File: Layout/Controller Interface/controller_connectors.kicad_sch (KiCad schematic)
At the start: 16 parts, among them J2 Controller 2, J3 Controller 3, J4 Controller 4, J7 Controller 1

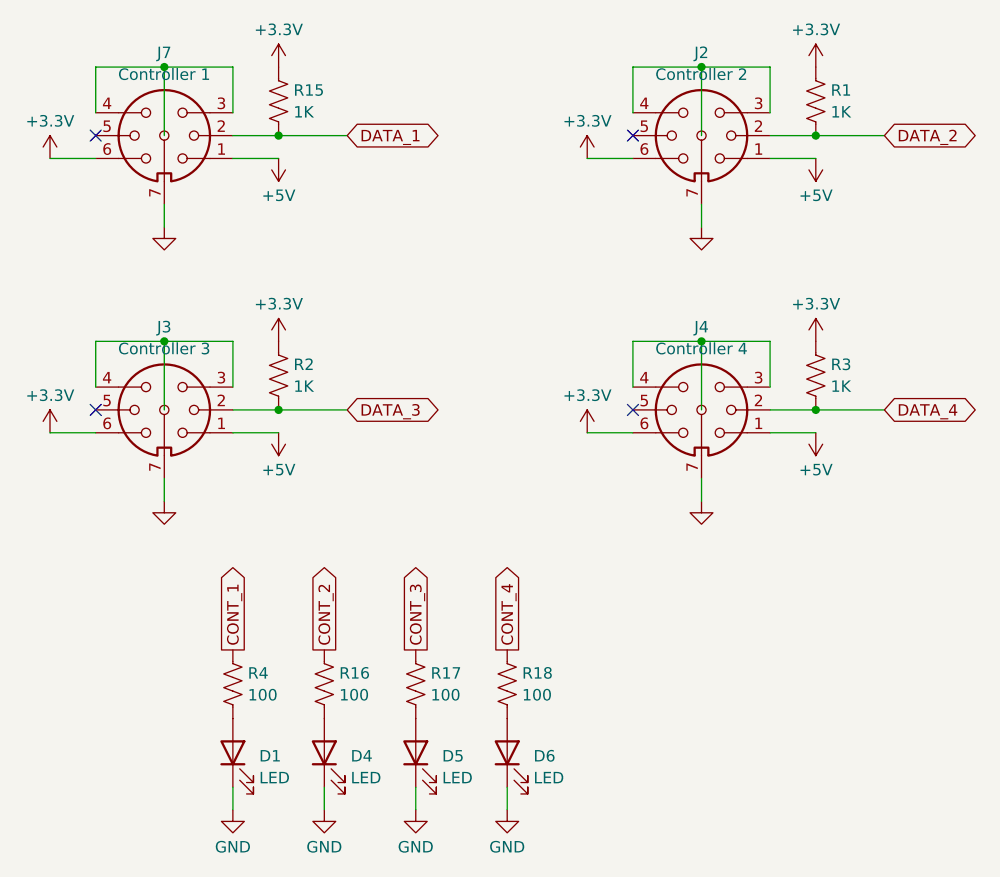
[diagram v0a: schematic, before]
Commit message: Completed schematic and layout
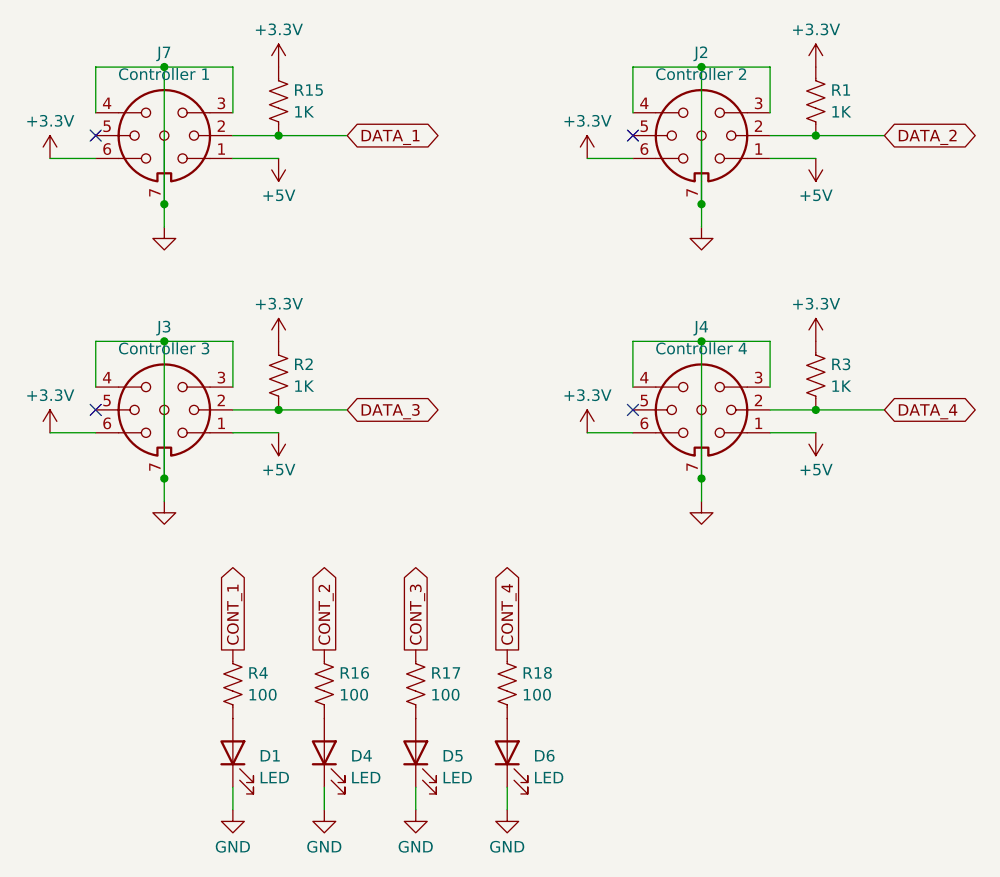
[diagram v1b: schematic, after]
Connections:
- net GND: now also J2.3, J2.4, J3.3, J3.4, J4.3, J4.4, J7.3, J7.4
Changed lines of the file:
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@@
 (kicad_sch (version 20230121) (generator eeschema)
   (paper "A4")
+  (junction (at 110.49 82.55) (diameter 0) (color 0 0 0 0)
+  )
+  (junction (at 170.18 82.55) (diameter 0) (color 0 0 0 0)
+  )
   (junction (at 123.19 105.41) (diameter 0) (color 0 0 0 0)
   )
-  (junction (at 170.18 97.79) (diameter 0) (color 0 0 0 0)
+  (junction (at 110.49 113.03) (diameter 0) (color 0 0 0 0)
   )
   (junction (at 110.49 97.79) (diameter 0) (color 0 0 0 0)
+  )
+  (junction (at 170.18 97.79) (diameter 0) (color 0 0 0 0)
   )
   (junction (at 110.49 67.31) (diameter 0) (color 0 0 0 0)
@@
   )
   (junction (at 170.18 67.31) (diameter 0) (color 0 0 0 0)
+  )
+  (junction (at 170.18 113.03) (diameter 0) (color 0 0 0 0)
   )
   (no_connect (at 102.87 105.41))
@@
     (stroke (width 0) (type default))
   )
-  (wire (pts (xy 110.49 67.31) (xy 118.11 67.31))
+  (wire (pts (xy 102.87 67.31) (xy 110.49 67.31))
     (stroke (width 0) (type default))
   )
@@
     (stroke (width 0) (type default))
   )
-  (wire (pts (xy 170.18 97.79) (xy 170.18 105.41))
-    (stroke (width 0) (type default))
-  )
   (wire (pts (xy 177.8 105.41) (xy 182.88 105.41))
     (stroke (width 0) (type default))
@@
     (stroke (width 0) (type default))
   )
-  (wire (pts (xy 110.49 97.79) (xy 118.11 97.79))
-    (stroke (width 0) (type default))
-  )
-  (wire (pts (xy 102.87 67.31) (xy 110.49 67.31))
+  (wire (pts (xy 102.87 97.79) (xy 110.49 97.79))
     (stroke (width 0) (type default))
   )
@@
     (stroke (width 0) (type default))
   )
-  (wire (pts (xy 110.49 67.31) (xy 110.49 74.93))
+  (wire (pts (xy 110.49 113.03) (xy 110.49 115.57))
+    (stroke (width 0) (type default))
+  )
+  (wire (pts (xy 110.49 67.31) (xy 118.11 67.31))
     (stroke (width 0) (type default))
   )
   (wire (pts (xy 118.11 147.32) (xy 118.11 149.86))
+    (stroke (width 0) (type default))
+  )
+  (wire (pts (xy 110.49 67.31) (xy 110.49 82.55))
     (stroke (width 0) (type default))
   )
@@
   )
   (wire (pts (xy 182.88 105.41) (xy 190.5 105.41))
-    (stroke (width 0) (type default))
-  )
-  (wire (pts (xy 170.18 67.31) (xy 170.18 74.93))
-    (stroke (width 0) (type default))
-  )
-  (wire (pts (xy 110.49 113.03) (xy 110.49 115.57))
     (stroke (width 0) (type default))
   )
@@
     (stroke (width 0) (type default))
   )
-  (wire (pts (xy 110.49 97.79) (xy 110.49 105.41))
-    (stroke (width 0) (type default))
-  )
   (wire (pts (xy 157.48 77.47) (xy 162.56 77.47))
     (stroke (width 0) (type default))
@@
     (stroke (width 0) (type default))
   )
-  (wire (pts (xy 118.11 97.79) (xy 118.11 102.87))
+  (wire (pts (xy 170.18 67.31) (xy 170.18 82.55))
     (stroke (width 0) (type default))
   )
-  (wire (pts (xy 102.87 97.79) (xy 110.49 97.79))
+  (wire (pts (xy 118.11 97.79) (xy 118.11 102.87))
     (stroke (width 0) (type default))
   )
@@
   )
   (wire (pts (xy 170.18 67.31) (xy 177.8 67.31))
+    (stroke (width 0) (type default))
+  )
+  (wire (pts (xy 110.49 97.79) (xy 118.11 97.79))
     (stroke (width 0) (type default))
   )
@@
     (stroke (width 0) (type default))
   )
+  (wire (pts (xy 170.18 97.79) (xy 170.18 113.03))
+    (stroke (width 0) (type default))
+  )
   (wire (pts (xy 177.8 74.93) (xy 182.88 74.93))
     (stroke (width 0) (type default))
@@
     (stroke (width 0) (type default))
   )
+  (wire (pts (xy 110.49 97.79) (xy 110.49 113.03))
+    (stroke (width 0) (type default))
+  )
